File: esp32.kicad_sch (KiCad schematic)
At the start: 37 parts, among them J2 USB_C_Receptacle_USB2.0, J3 Conn_ARM_JTAG_SWD_10, J4 SBC1_UART, J5 SBC2_UART, Q2 BC846, Q3 BC846, SW1 SW_Push, SW2 SW_Push, U3 MCP7940N-xMNY, U4 USB6B1, U5 CP2102N-Axx-xQFN24, U6 ESP32-WROOM-32D, Y1 32.768 kHz

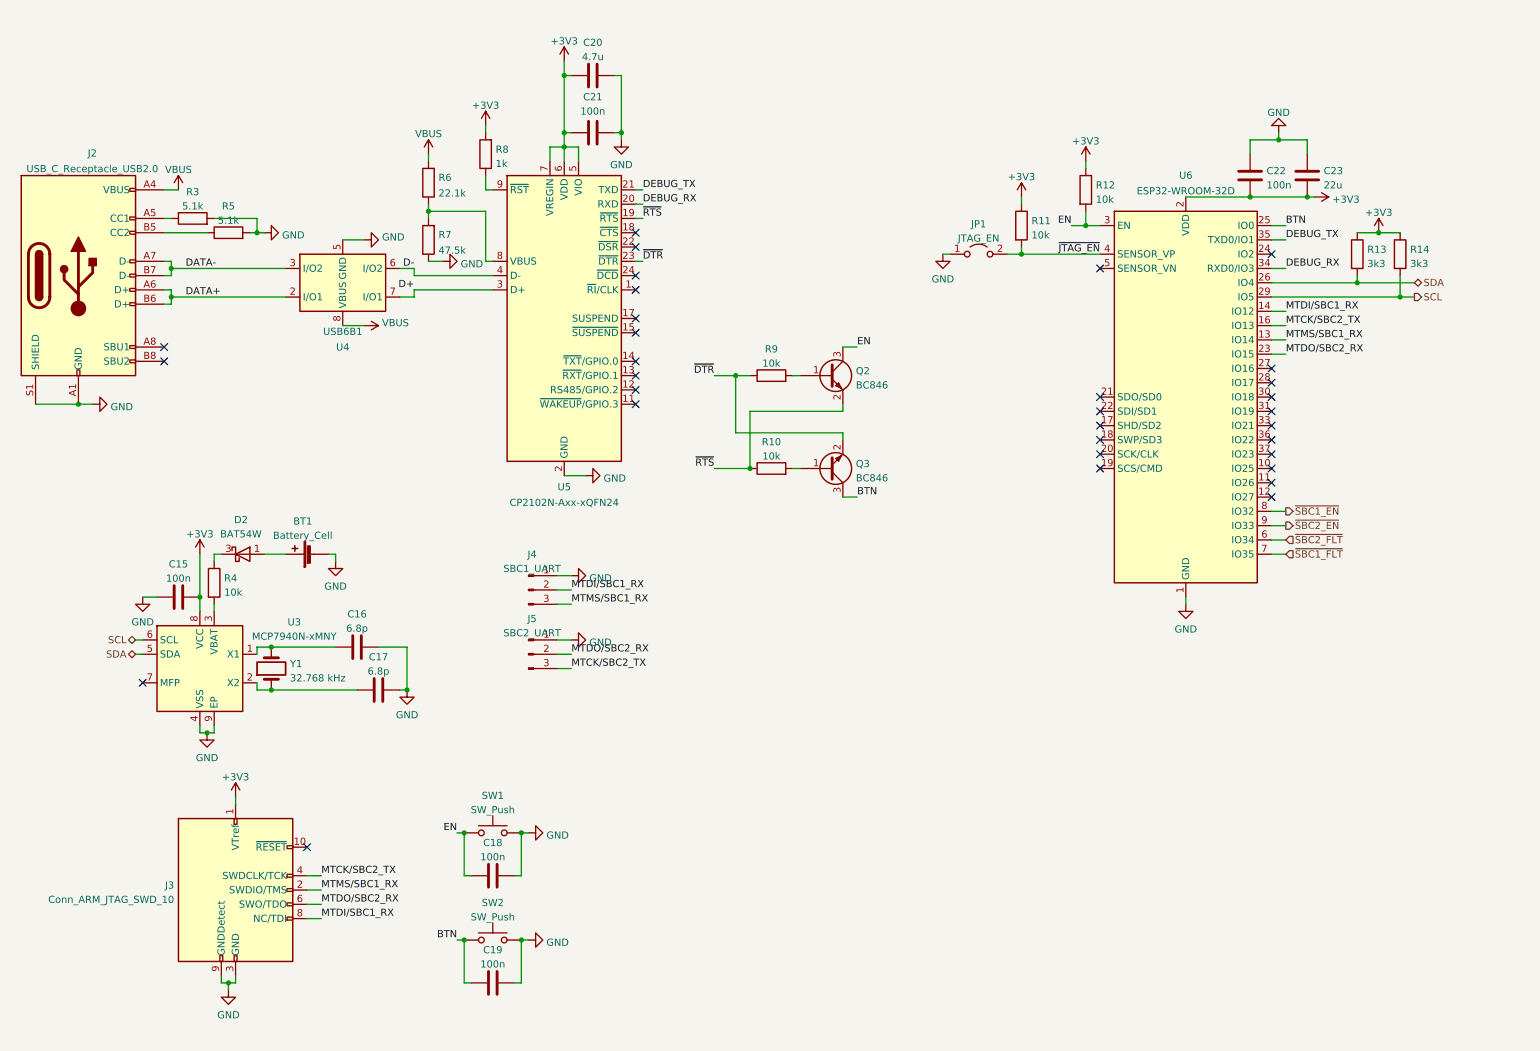
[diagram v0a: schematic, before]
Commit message: Second revision
Signed-off-by: Roman Ondráček <ondracek.roman@centrum.cz>
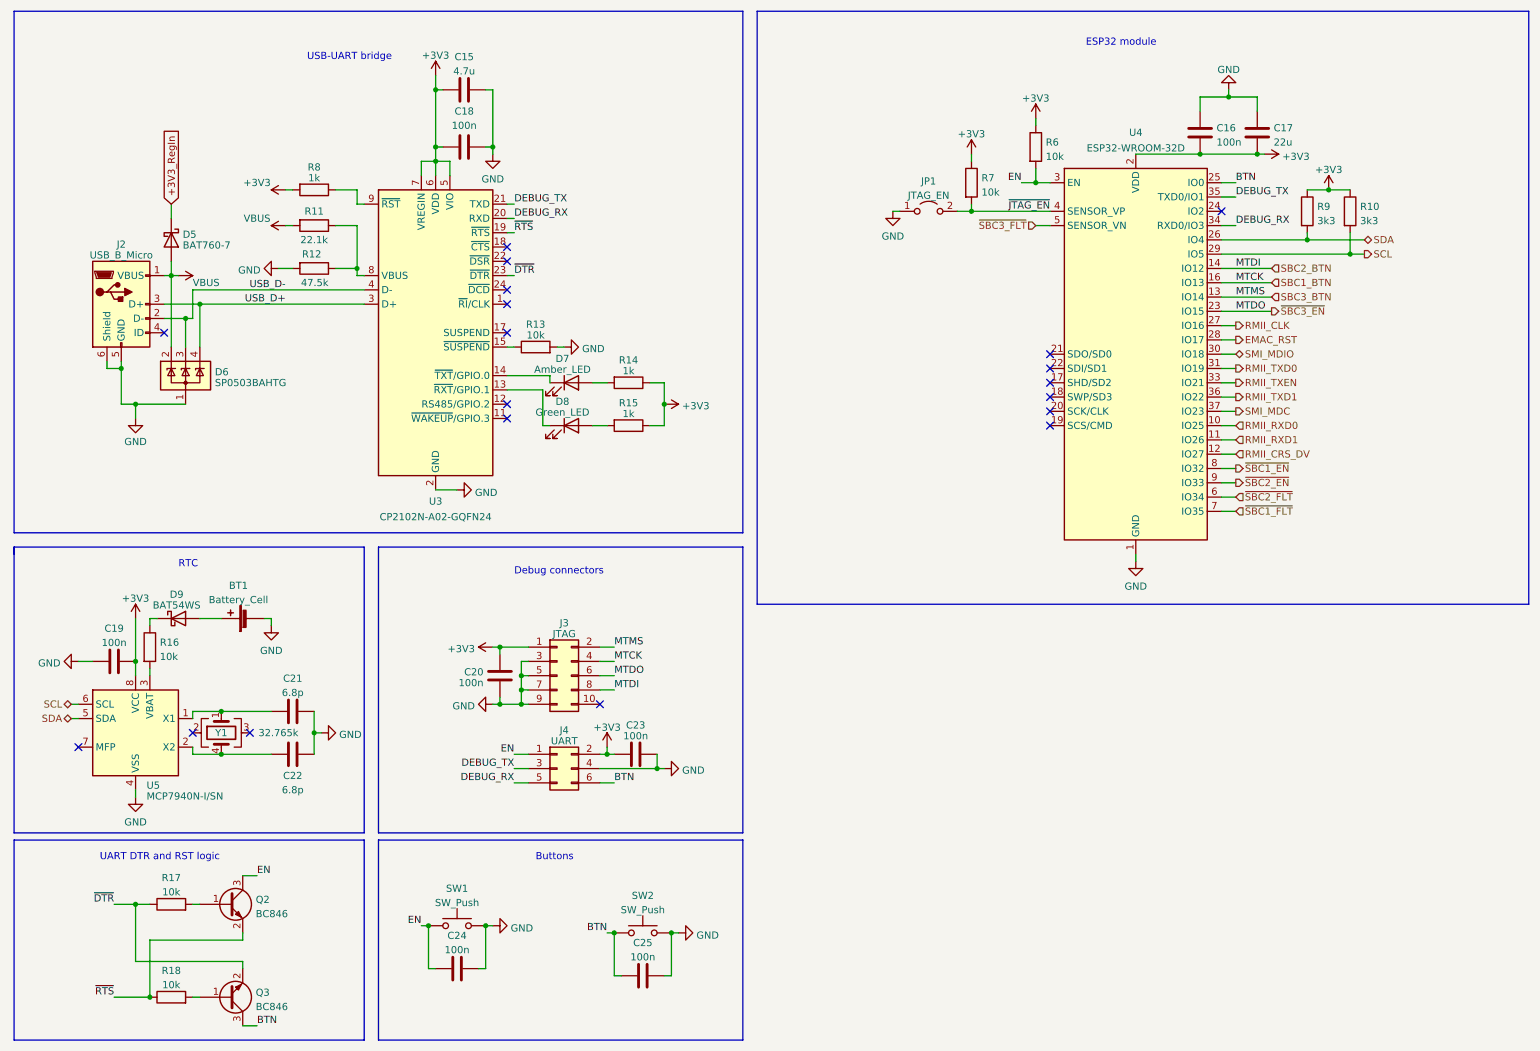
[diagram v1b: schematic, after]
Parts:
- removed D2: BAT54W, Package_TO_SOT_SMD:SOT-323_SC-70, symbol Diode:BAT54W
- removed J2: USB_C_Receptacle_USB2.0, Connector_USB:USB_C_Receptacle_JAE_DX07S016JA1R1500, symbol Connector:USB_C_Receptacle_USB2.0
- removed J3: Conn_ARM_JTAG_SWD_10, Connector_IDC:IDC-Header_2x05_P2.54mm_Vertical, symbol Connector:Conn_ARM_JTAG_SWD_10
- removed J4: SBC1_UART, Connector_PinHeader_2.54mm:PinHeader_1x03_P2.54mm_Vertical, symbol Connector:Conn_01x03_Male
- removed J5: SBC2_UART, Connector_PinHeader_2.54mm:PinHeader_1x03_P2.54mm_Vertical, symbol Connector:Conn_01x03_Male
- removed R3, R5: 5.1k, Resistor_SMD:R_0402_1005Metric_Pad0.72x0.64mm_HandSolder, symbol Device:R
- removed U3: MCP7940N-xMNY, Package_DFN_QFN:DFN-8-1EP_3x2mm_P0.5mm_EP1.36x1.46mm, symbol Timer_RTC:MCP7940N-xMNY
- removed U4: USB6B1, Package_SO:SOIC-8_3.9x4.9mm_P1.27mm, symbol Power_Protection:USB6B1
- removed Y1: 32.768 kHz, Crystal:Crystal_SMD_G8-2Pin_3.2x1.5mm_HandSoldering, symbol Device:Crystal
- added C20, C23: 100n, Capacitor_SMD:C_0402_1005Metric_Pad0.74x0.62mm_HandSolder, symbol Device:C
- added D5: BAT760-7, Diode_SMD:D_SOD-323_HandSoldering, symbol Device:D_Schottky
- added D6: SP0503BAHTG, Package_TO_SOT_SMD:SOT-143, symbol Power_Protection:SP0503BAHT
- added D7: Amber_LED, LED_SMD:LED_0603_1608Metric_Pad1.05x0.95mm_HandSolder, symbol Device:LED
- added D8: Green_LED, LED_SMD:LED_0603_1608Metric_Pad1.05x0.95mm_HandSolder, symbol Device:LED
- added D9: BAT54WS, Diode_SMD:D_SOD-323_HandSoldering, symbol Device:D_Schottky
- added J2: USB_B_Micro, Connector_USB:USB_Micro-B_GCT_USB3076-30-A, symbol Connector:USB_B_Micro
- added J3: JTAG, Connector_IDC:IDC-Header_2x05_P2.54mm_Vertical, symbol Connector_Generic:Conn_02x05_Odd_Even
- added J4: UART, Connector_IDC:IDC-Header_2x03_P2.54mm_Vertical, symbol Connector_Generic:Conn_02x03_Odd_Even
- added R13: 10k, Resistor_SMD:R_0402_1005Metric_Pad0.72x0.64mm_HandSolder, symbol Device:R
- added R14, R15: 1k, Resistor_SMD:R_0402_1005Metric_Pad0.72x0.64mm_HandSolder, symbol Device:R
- added U5: MCP7940N-I/SN, Package_SO:SOIC-8_3.9x4.9mm_P1.27mm, symbol Timer_RTC:MCP7940N-xSN
- added Y1: 32.765k, Crystal:Crystal_SMD_Abracon_ABS25-4Pin_8.0x3.8mm, symbol Device:Crystal_GND23
- BT1: Mouser (none) -> https://cz.mouser.com/ProductDetail/534-3034
- C15: renamed from C20; Mouser (none) -> https://cz.mouser.com/ProductDetail/81-GRM31CR71H475KA2K
- C16: renamed from C22; Mouser (none) -> https://cz.mouser.com/ProductDetail/187-CL21B104KCFSFNE
- C17: renamed from C23; Mouser (none) -> https://cz.mouser.com/ProductDetail/187-CL31A226MOCLNNC
- C19: renamed from C15; Mouser (none) -> https://cz.mouser.com/ProductDetail/187-CL21B104KCFSFNE
- C21: renamed from C16; value C -> 6.8p; Mouser (none) -> https://cz.mouser.com/ProductDetail/81-GRM1555C1H6R8DA1D
- C22: renamed from C17; value C -> 6.8p; Mouser (none) -> https://cz.mouser.com/ProductDetail/81-GRM1555C1H6R8DA1D
- C24: renamed from C18; Mouser (none) -> https://cz.mouser.com/ProductDetail/187-CL21B104KCFSFNE
- C25: renamed from C19; Mouser (none) -> https://cz.mouser.com/ProductDetail/187-CL21B104KCFSFNE
- Q2, Q3: Mouser (none) -> https://cz.mouser.com/ProductDetail/771-BC846BW135
- R10: renamed from R14; Mouser (none) -> https://cz.mouser.com/ProductDetail/603-RC0402FR-073K3L
- R11: renamed from R6; Mouser (none) -> https://cz.mouser.com/ProductDetail/603-RC0402FR-1322K1L
- R12: renamed from R7; Mouser (none) -> https://cz.mouser.com/ProductDetail/603-RC0402FR-1047K5L
- R16: renamed from R4; Mouser (none) -> https://cz.mouser.com/ProductDetail/652-CR0402FX-1002GLF
- R17: renamed from R9; Mouser (none) -> https://cz.mouser.com/ProductDetail/652-CR0402FX-1002GLF
- R18: renamed from R10; Mouser (none) -> https://cz.mouser.com/ProductDetail/652-CR0402FX-1002GLF
- R6: renamed from R12; Mouser (none) -> https://cz.mouser.com/ProductDetail/652-CR0402FX-1002GLF
- R7: renamed from R11; Mouser (none) -> https://cz.mouser.com/ProductDetail/652-CR0402FX-1002GLF
- R8: Mouser (none) -> https://cz.mouser.com/ProductDetail/603-RC0402FR-071KL
- R9: renamed from R13; Mouser (none) -> https://cz.mouser.com/ProductDetail/603-RC0402FR-073K3L
- U3: renamed from U5; value CP2102N-Axx-xQFN24 -> CP2102N-A02-GQFN24
- U4: renamed from U6; Mouser https://cz.mouser.com/ProductDetail/356-ES32WROOM32D16MB -> https://cz.mouser.com/ProductDetail/356-ESP32WRM32E128PH
- renumbered C21 to C18
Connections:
- net +3V3: now also C20.1, C23.1, J3.1 (Pin_1), J4.2 (Pin_2), R14.1, R15.1, U5.8 (VCC)
- net BTN: now also J4.6 (Pin_6)
- net DEBUG_RX: now also J4.5 (Pin_5)
- net DEBUG_TX: now also J4.3 (Pin_3)
- net EN: now also J4.1 (Pin_1)
- net GND: now also R12.2, C20.2, C23.2, D6.1 (A), J2.5 (GND), J2.6 (Shield), J3.3 (Pin_3), J3.5 (Pin_5), J3.7 (Pin_7), J3.9 (Pin_9), J4.4 (Pin_4), R13.2, U5.4 (VSS); no longer R12.1
- net SCL: now also U5.6 (SCL)
- net SDA: now also U5.5 (SDA)
- net VBUS: now also D5.2 (A), D6.2 (K), J2.1 (VBUS)
- net at C22.1: now also U5.2 (X2), Y1.4
- net at C21.1: now also U5.1 (X1), Y1.1
- net at R16.2: now also U5.3 (VBAT)
- net at R11.1, U3.8 (VBUS): now also R12.1; no longer R12.2
- net at U3.13 (~{RXT}/GPIO.1): now also D8.1 (K)
- net at U3.14 (~{TXT}/GPIO.0): now also D7.1 (K)
- net at U3.15 (~{SUSPEND}): now also R13.1
- net at BT1.1 (+): now also D9.2 (A)
- net at R16.1: now also D9.1 (K)
- net RMII_RXD0: now reaches U4.10 (IO25)
- net RMII_RXD1: now reaches U4.11 (IO26)
- net RMII_CRS_DV: now reaches U4.12 (IO27)
- net RMII_CLK: now reaches U4.27 (IO16)
- net EMAC_RST: now reaches U4.28 (IO17)
- net SMI_MDIO: now reaches U4.30 (IO18)
- net RMII_TXD0: now reaches U4.31 (IO19)
- net RMII_TXEN: now reaches U4.33 (IO21)
- net RMII_TXD1: now reaches U4.36 (IO22)
- net SMI_MDC: now reaches U4.37 (IO23)
- net ~{SBC3_FLT}: now reaches U4.5 (SENSOR_VN)
- net D+ renamed USB_D+
- net USB_D+: now also D6.4 (K), J2.3 (D+)
- net D- renamed USB_D-
- net USB_D-: now also D6.3 (K), J2.2 (D-)
- net MTCK/SBC2_TX renamed SBC1_BTN
- net SBC1_BTN: now also J3.4 (Pin_4)
- net MTDI/SBC1_RX renamed SBC2_BTN
- net SBC2_BTN: now also J3.8 (Pin_8)
- net MTDO/SBC2_RX renamed ~{SBC3_EN}
- net ~{SBC3_EN}: now also J3.6 (Pin_6)
- net MTMS/SBC1_RX renamed SBC3_BTN
- net SBC3_BTN: now also J3.2 (Pin_2)
- new net: D8.2 (A), R15.2
- new net: D7.2 (A), R14.2
- new net +3V3_RegIn: D5.1 (K)
- no-connect marks 32 -> 19
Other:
- note added: "Buttons"
- note added: "Debug connectors"
- note added: "ESP32 module"
- note added: "RTC"
- note added: "UART DTR and RST logic"
- note added: "USB-UART bridge"
- title: (none) -> PDU with Consumption Metering Function for SBCs
- moved on the sheet: BT1, C15, C16, C17, C18, C19, C21, C22, C24, C25, JP1, Q2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
